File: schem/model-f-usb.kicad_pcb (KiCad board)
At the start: 2 copper layers, 127 x 28.2 mm, 79 parts, among them P1 CONN_5, P2 CONN_3X2, SW1 SW_PUSH, SW2 SW_PUSH, U1 ATMEGA32U2, U2 DAC101S101, U3 LM339A, U4 LM339A, U5 74AHC595, U6 74AHC595, X1 16MHz

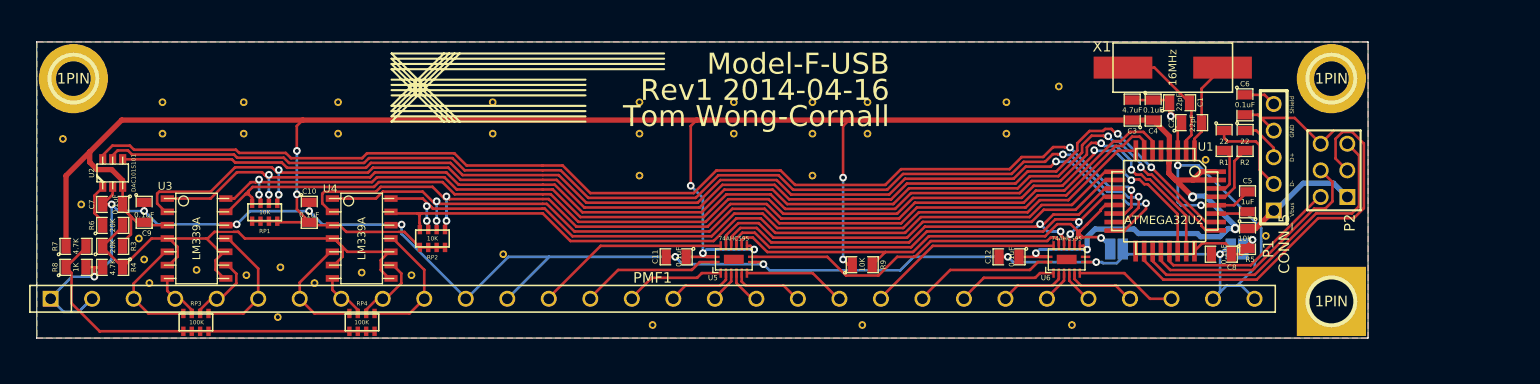
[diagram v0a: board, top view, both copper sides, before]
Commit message: 0.6.7, imported from xwhatit's untracked source code
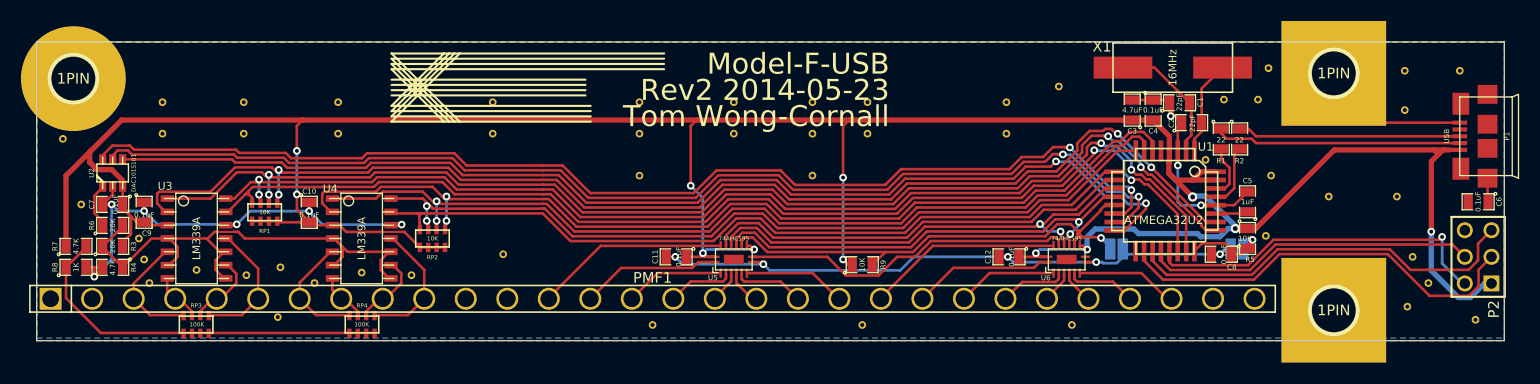
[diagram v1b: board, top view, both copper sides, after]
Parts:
- removed the 1PIN at (279.2, 180.2)
- removed the 1PIN at (279.2, 201.5)
- added .: ., Via, F.Cu at (287.0, 197.2)
- added .: ., Via, F.Cu at (288.5, 199.8)
- added .: ., Via, F.Cu at (279.0, 191.5)
- added .: ., Via, F.Cu at (285.5, 191.5)
- added .: ., Via, F.Cu at (286.2, 179.5)
- added .: ., Via, F.Cu at (291.5, 179.5)
- added .: ., Via, F.Cu at (286.2, 183.2)
- added .: ., Via, F.Cu at (272.2, 182.2)
- added .: ., Via, F.Cu at (269.0, 182.2)
- added .: ., Via, F.Cu at (273.2, 179.2)
- added .: ., Via, F.Cu at (273.5, 189.5)
- added .: ., Via, F.Cu at (286.5, 202.0)
- added .: ., Via, F.Cu at (293.0, 203.2)
- added 1PIN: P***, 1pin, F.Cu at (279.5, 179.8)
- added 1PIN: P***, 1pin, F.Cu at (279.5, 202.3)
- P1: value CONN_5 -> USB; footprint PIN_ARRAY_5x1 -> USB-Micro-B-SMT
- PMF1: footprint PIN_ARRAY_3_96-30X1 -> PIN_ARRAY_3_96-30X1_large_pads
- SW1: value SW_PUSH -> PROG
- SW2: value SW_PUSH -> RESET
- moved C6 24.1 mm to (293.2, 192.0), turned to 180 degrees
- moved P1 17.9 mm to (291.5, 185.8)
- moved P2 16.0 mm to (293.2, 197.2)
- moved R2 0.54 mm to (270.5, 186.0)
- moved R1 0.31 mm to (268.8, 186.0)
- moved RP3 0.20 mm to (171.0, 203.7)
- moved RP4 0.20 mm to (186.8, 203.7)
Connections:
- P1 pad 4: GND -> (no net)
- P1 pad 5: /USB_SHIELD -> GND
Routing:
- net GND: track 214.4 -> 143.1 mm
- net VCC: track 262.6 -> 294.0 mm, vias 11 -> 12
- net /USB_D+: track 4.31 -> 21.3 mm
- net N-0000015: track 18.3 -> 33.8 mm, vias 0 -> 1
- net /USB_D-: track 8.63 -> 23.6 mm
- net N-000003: track 23.8 -> 31.8 mm
- net N-000004: track 30.3 -> 38.1 mm
- net N-000005: track 38.5 -> 39.9 mm
- net /USB_SHIELD: track 3.11 -> 2.27 mm
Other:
- board size 127 x 28.2 mm -> 140 x 28.5 mm
- board text added: "Rev2 2014-05-23"
- board text removed: "D+"
- board text removed: "D-"
- board text removed: "GND"
- board text removed: "Rev1 2014-04-16"
- board text removed: "Shield"
- board text removed: "Vbus"
